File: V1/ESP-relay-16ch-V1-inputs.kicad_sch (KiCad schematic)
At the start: 80 parts, among them U1 LTV-817S, U10 LTV-817S, U11 LTV-817S, U12 LTV-817S, U13 LTV-817S, U14 LTV-817S, U15 LTV-817S, U16 LTV-817S, U2 LTV-817S, U3 LTV-817S, U4 LTV-817S, U5 LTV-817S, U6 LTV-817S, U7 LTV-817S, U8 LTV-817S, U9 LTV-817S

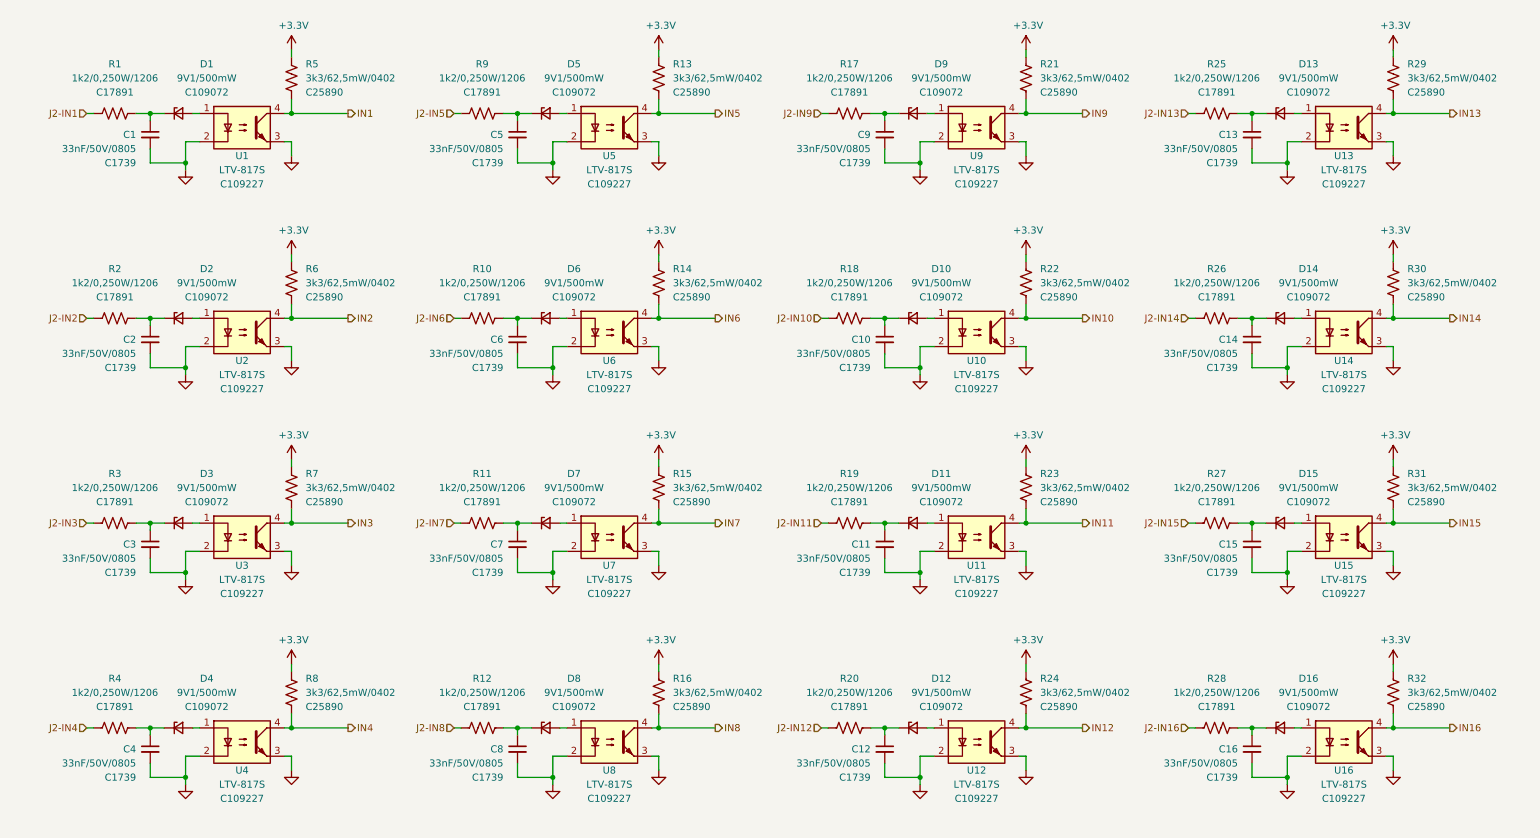
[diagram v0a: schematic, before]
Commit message: Dev updates
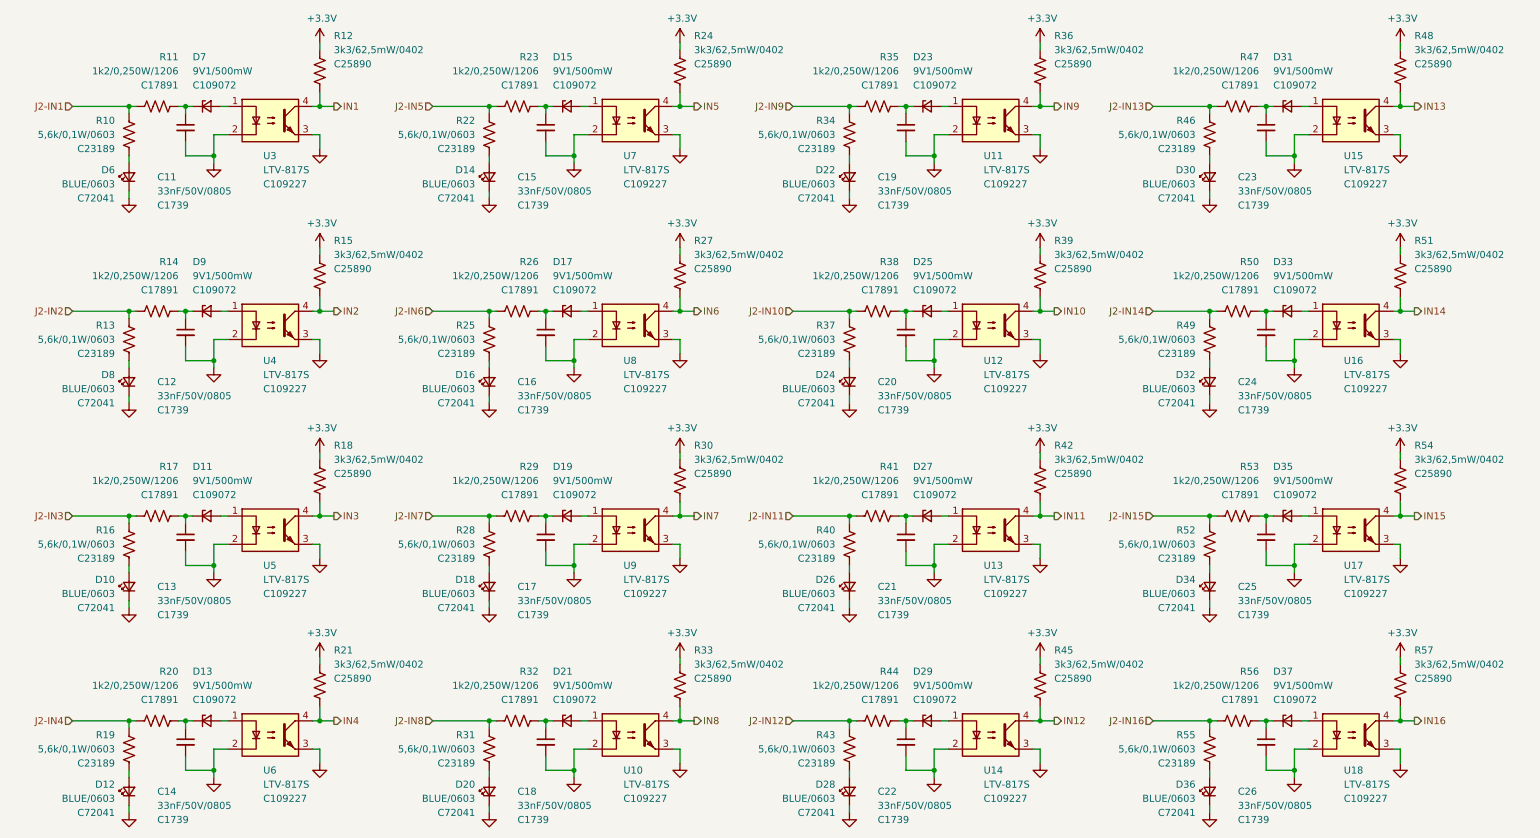
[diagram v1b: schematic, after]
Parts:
- removed C1, C10, C2, C3, C4, C5, C6, C7, C8, C9: 33nF/50V/0805, Tales:C_0805_2012Metric, symbol Device:C_Small
- removed D1, D10, D12, D14, D16, D2, D3, D4, D5, D6, D8: 9V1/500mW, Tales:D_MiniMELF, symbol Device:D_Zener_Small
- removed R1, R2, R3, R4, R9: 1k2/0,250W/1206, Tales:R_1206_3216Metric, symbol Device:R_US
- removed R5, R6, R7, R8: 3k3/62,5mW/0402, Tales:R_0402_1005Metric, symbol Device:R_US
- removed U1, U2: LTV-817S, Tales:SMDIP-4_W9.53mm, symbol Isolator:LTV-817S
- added C17, C18, C19, C20, C21, C22, C23, C24, C25, C26: 33nF/50V/0805, Tales:C_0805_2012Metric, symbol Device:C_Small
- added D10, D12, D14, D16, D18, D20, D22, D24, D26, D28, D30, D32, D34, D36, D6, D8: BLUE/0603, Tales:LED_0603_1608Metric, symbol Device:LED_Small
- added D17, D19, D21, D23, D25, D27, D29, D31, D33, D35, D37: 9V1/500mW, Tales:D_MiniMELF, symbol Device:D_Zener_Small
- added R33, R36, R39, R42, R45, R48, R51, R54, R57: 3k3/62,5mW/0402, Tales:R_0402_1005Metric, symbol Device:R_US
- added R34, R37, R40, R43, R46, R49, R52, R55: 5,6k/0,1W/0603, Tales:R_0603_1608Metric, symbol Device:R_US
- added R35, R38, R41, R44, R47, R50, R53, R56: 1k2/0,250W/1206, Tales:R_1206_3216Metric, symbol Device:R_US
- added U17, U18: LTV-817S, Tales:SMDIP-4_W9.53mm, symbol Isolator:LTV-817S
- R10, R19, R25, R28: value 1k2/0,250W/1206 -> 5,6k/0,1W/0603; footprint Tales:R_1206_3216Metric -> Tales:R_0603_1608Metric; Case 1206/3216 -> 0603/1608; LCSC Part # C17891 -> C23189; Mfr PN 1206W4F1201T5E -> 0603WAF5601T5E; Vendor PN C17891 -> C23189
- R12, R18, R27: value 1k2/0,250W/1206 -> 3k3/62,5mW/0402; footprint Tales:R_1206_3216Metric -> Tales:R_0402_1005Metric; Case 1206/3216 -> 0402/1005; LCSC Part # C17891 -> C25890; Mfr PN 1206W4F1201T5E -> 0402WGF3301TCE; Vendor PN C17891 -> C25890
- R13, R16, R22, R31: value 3k3/62,5mW/0402 -> 5,6k/0,1W/0603; footprint Tales:R_0402_1005Metric -> Tales:R_0603_1608Metric; Case 0402/1005 -> 0603/1608; LCSC Part # C25890 -> C23189; Mfr PN 0402WGF3301TCE -> 0603WAF5601T5E; Vendor PN C25890 -> C23189
- R14, R23, R29, R32: value 3k3/62,5mW/0402 -> 1k2/0,250W/1206; footprint Tales:R_0402_1005Metric -> Tales:R_1206_3216Metric; Case 0402/1005 -> 1206/3216; LCSC Part # C25890 -> C17891; Mfr PN 0402WGF3301TCE -> 1206W4F1201T5E; Vendor PN C25890 -> C17891
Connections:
- net +3.3V: now also R12.1, R18.1, R27.1, R33.1, R36.1, R39.1, R42.1, R45.1, R48.1, R51.1, R54.1, R57.1; no longer R13.1, R14.1, R16.1, R22.1, R23.1, R29.1, R31.1, R32.1
- net GND: now also C17.2, C18.2, C19.2, C20.2, C21.2, C22.2, C23.2, C24.2, C25.2, C26.2, D10.1 (K), D12.1 (K), D14.1 (K), D16.1 (K), D18.1 (K), D20.1 (K), D22.1 (K), D24.1 (K), D26.1 (K), D28.1 (K), D30.1 (K), D32.1 (K), D34.1 (K), D36.1 (K), D6.1 (K), D8.1 (K), U17.2, U17.3, U18.2, U18.3
- net IN1: now also R12.2, U3.4
- net IN10: now also U12.4, R39.2; no longer R22.2, U10.4
- net IN11: now also U13.4, R42.2; no longer R23.2, U11.4
- net IN12: now also U14.4, R45.2; no longer R24.2, U12.4
- net IN13: now also U15.4, R48.2; no longer R29.2, U13.4
- net IN14: now also U16.4, R51.2; no longer R30.2, U14.4
- net IN15: now also R54.2, U17.4; no longer R31.2, U15.4
- net IN16: now also R57.2, U18.4; no longer R32.2, U16.4
- net IN2: now also R15.2, U4.4
- net IN3: now also R18.2, U5.4; no longer U3.4
- net IN4: now also R21.2, U6.4; no longer U4.4
- net IN5: now also R24.2, U7.4; no longer R13.2, U5.4
- net IN6: now also R27.2, U8.4; no longer R14.2, U6.4
- net IN7: now also R30.2, U9.4; no longer R15.2, U7.4
- net IN8: now also U10.4, R33.2; no longer R16.2, U8.4
- net IN9: now also U11.4, R36.2; no longer R21.2, U9.4
- net J2-IN1: now also R10.1, R11.2
- net J2-IN10: now also R37.1, R38.2; no longer R18.2
- net J2-IN11: now also R40.1, R41.2; no longer R19.2
- net J2-IN12: now also R43.1, R44.2; no longer R20.2
- net J2-IN13: now also R46.1, R47.2; no longer R25.2
- net J2-IN14: now also R49.1, R50.2; no longer R26.2
- net J2-IN15: now also R52.1, R53.2; no longer R27.2
- net J2-IN16: now also R55.1, R56.2; no longer R28.2
- net J2-IN2: now also R13.1, R14.2
- net J2-IN3: now also R16.1, R17.2
- net J2-IN4: now also R19.1, R20.2
- net J2-IN5: now also R22.1, R23.2
- net J2-IN6: now also R25.1, R26.2; no longer R10.2
- net J2-IN7: now also R28.1, R29.2; no longer R11.2
- net J2-IN8: now also R31.1, R32.2; no longer R12.2
- net J2-IN9: now also R34.1, R35.2; no longer R17.2
- net at R17.1: now also C13.1, D11.1 (K); no longer D9.1 (K)
- net at U9.1: now also D19.2 (A); no longer D9.2 (A)
- net at U6.1: now also D13.2 (A)
- net at C14.1: now also D13.1 (K), R20.1; no longer R26.1
- net at U14.1: now also D29.2 (A)
- net at U8.1: now also D17.2 (A)
- net at U10.1: now also D21.2 (A)
- net at U16.1: now also D33.2 (A)
- net at U4.1: now also D9.2 (A)
- net at C12.1: now also D9.1 (K), R14.1; no longer R20.1
- net at U11.1: now also D23.2 (A); no longer D11.2 (A)
- net at C16.1: now also R26.1, D17.1 (K); no longer R28.1
- net at C15.1, D15.1 (K): now also R23.1; no longer R27.1
- net at U12.1: now also D25.2 (A)
- net at U15.1: now also D31.2 (A); no longer D15.2 (A)
- net at U5.1: now also D11.2 (A)
- net at D7.1 (K), R11.1: now also C11.1
- net at D7.2 (A): now also U3.1; no longer U7.1
- net at U13.1: now also D27.2 (A); no longer D13.2 (A)
- new net: D18.2 (A), R28.2
- new net: C21.1, D27.1 (K), R41.1
- new net: D10.2 (A), R16.2
- new net: C26.1, D37.1 (K), R56.1
- new net: C23.1, D31.1 (K), R47.1
- new net: C18.1, D21.1 (K), R32.1
- new net: D34.2 (A), R52.2
- new net: D15.2 (A), U7.1
- new net: D12.2 (A), R19.2
- new net: D14.2 (A), R22.2
- new net: D16.2 (A), R25.2
- new net: C17.1, D19.1 (K), R29.1
- new net: C20.1, D25.1 (K), R38.1
- new net: D32.2 (A), R49.2
- new net: D6.2 (A), R10.2
- new net: C25.1, D35.1 (K), R53.1
- new net: C24.1, D33.1 (K), R50.1
- new net: D20.2 (A), R31.2
- new net: D26.2 (A), R40.2
- new net: D37.2 (A), U18.1
- new net: C22.1, D29.1 (K), R44.1
- new net: D22.2 (A), R34.2
- new net: D35.2 (A), U17.1
- new net: D24.2 (A), R37.2
- new net: C19.1, D23.1 (K), R35.1
- new net: D28.2 (A), R43.2
- new net: D30.2 (A), R46.2
- new net: D36.2 (A), R55.2
- new net: D8.2 (A), R13.2
